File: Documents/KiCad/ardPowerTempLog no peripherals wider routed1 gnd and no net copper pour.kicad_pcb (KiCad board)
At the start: 2 copper layers, 68.6 x 53.3 mm, 26 parts, among them J10 5-pin_3-pole_3,5mm_audio_head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, J11 4-pin_3LED_header, J12 Conn_01x02_Male, J13 Conn_01x02_Male, J6 5-pin_3-pole_3,5mm_audio_head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, J7 5-pin_3-pole_3,5mm_audio_head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, J8 5-pin_3-pole_3,5mm_audio_head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, J9 5-pin_3-pole_3,5mm_audio_head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

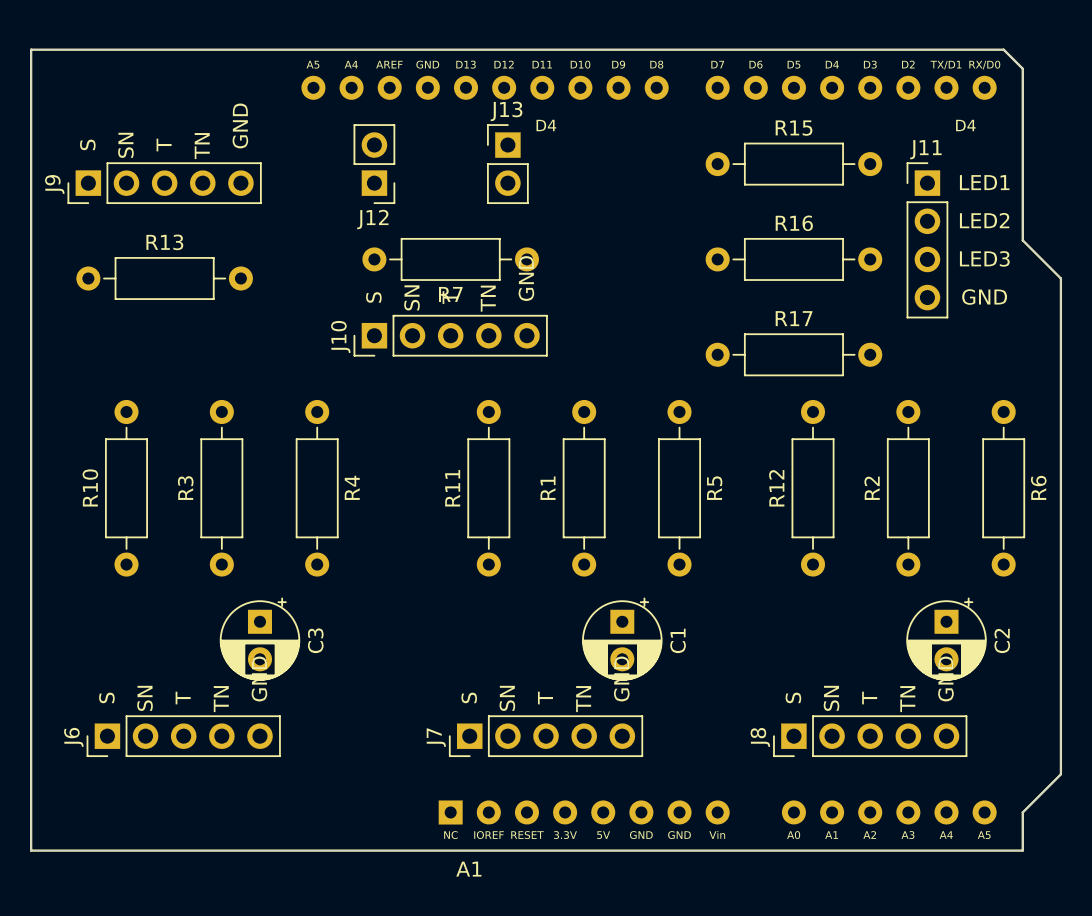
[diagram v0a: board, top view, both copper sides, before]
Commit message: schematics
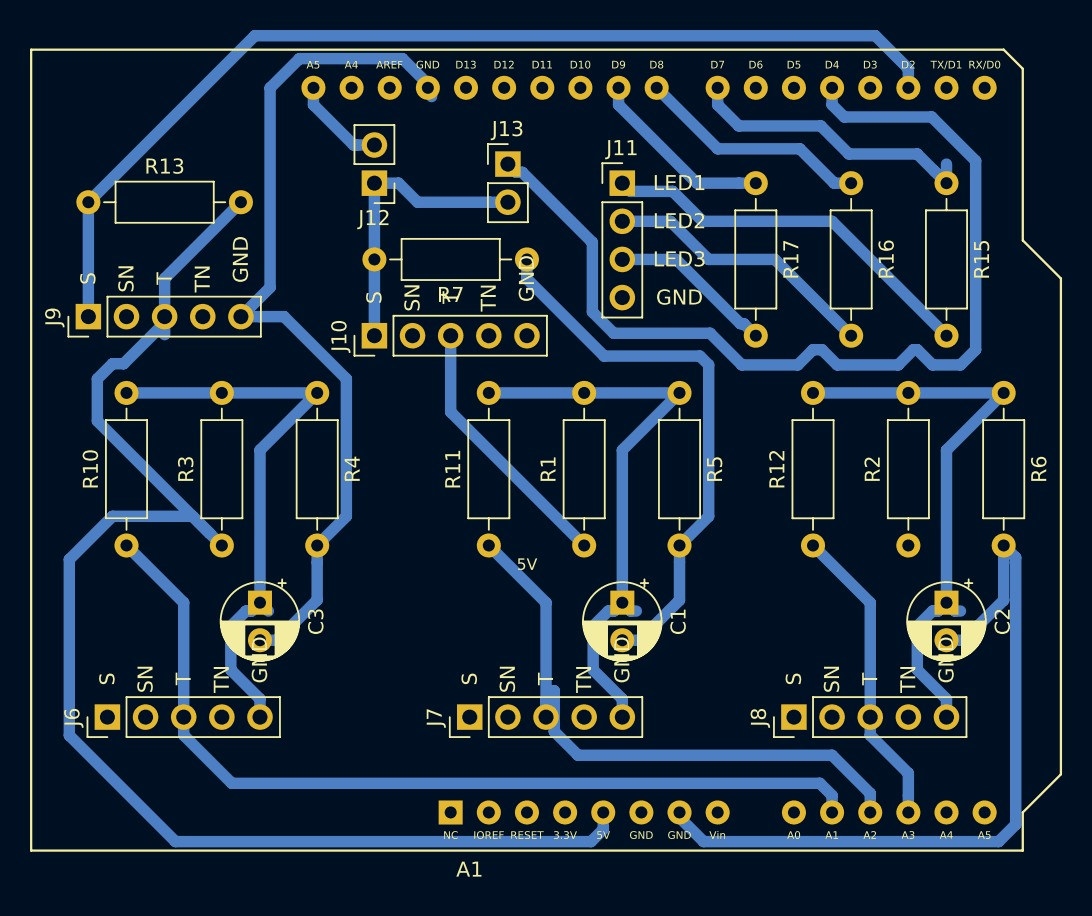
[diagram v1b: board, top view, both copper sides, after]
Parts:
- moved J11 20.3 mm to (144.8, 67.3)
- moved R15 15.3 mm to (166.4, 67.3), turned to 270 degrees
- moved R17 11.7 mm to (153.7, 67.3), turned to 270 degrees
- moved R16 10.2 mm to (160.0, 67.3), turned to 270 degrees
- moved J9 8.89 mm to (109.2, 76.2)
- moved R13 5.08 mm to (109.2, 68.6)
- moved J13 1.27 mm to (137.2, 66.0)
- moved C1 1.27 mm to (144.8, 95.2)
- moved C2 1.27 mm to (166.4, 95.2)
- moved C3 1.27 mm to (120.7, 95.2)
- moved J6 1.27 mm to (110.5, 102.9)
- moved J7 1.27 mm to (134.6, 102.9)
- moved J8 1.27 mm to (156.2, 102.9)
- moved R1 1.27 mm to (142.2, 91.4)
- moved R10 1.27 mm to (111.8, 91.4)
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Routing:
- net /GND: track 0.00 -> 146.7 mm
- net /Collector: track 0.00 -> 112.7 mm
- net /Data: track 0.00 -> 69.0 mm
- net Net-(A1-Pad19): track 0.00 -> 66.3 mm
- net Net-(A1-Pad10): track 0.00 -> 60.2 mm
- net Net-(A1-Pad11): track 0.00 -> 41.7 mm
- net Net-(C2-Pad1): track 0.00 -> 38.9 mm
- net Net-(C1-Pad1): track 0.00 -> 38.9 mm
- net Net-(C3-Pad1): track 0.00 -> 38.5 mm
- net Net-(D1-Pad2): track 0.00 -> 25.8 mm
- net Net-(A1-Pad12): track 0.00 -> 20.4 mm
- net Net-(A1-Pad22): track 0.00 -> 19.8 mm
- net /Emitter: track 0.00 -> 19.6 mm
- net Net-(D2-Pad2): track 0.00 -> 18.4 mm
- net Net-(A1-Pad23): track 0.00 -> 15.6 mm
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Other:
- board outline removed
- net class 30 added: clearance 0.762, trace_width 0.762, via_dia 2.032, via_drill 0.762
- board text added: "5V"
- board text removed: "D4"
